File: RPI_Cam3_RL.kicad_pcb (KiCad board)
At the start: 2 copper layers, 106 x 106 mm, 42 parts, among them J1 in, Q1 2N7002, U1 RPI_CAM_3

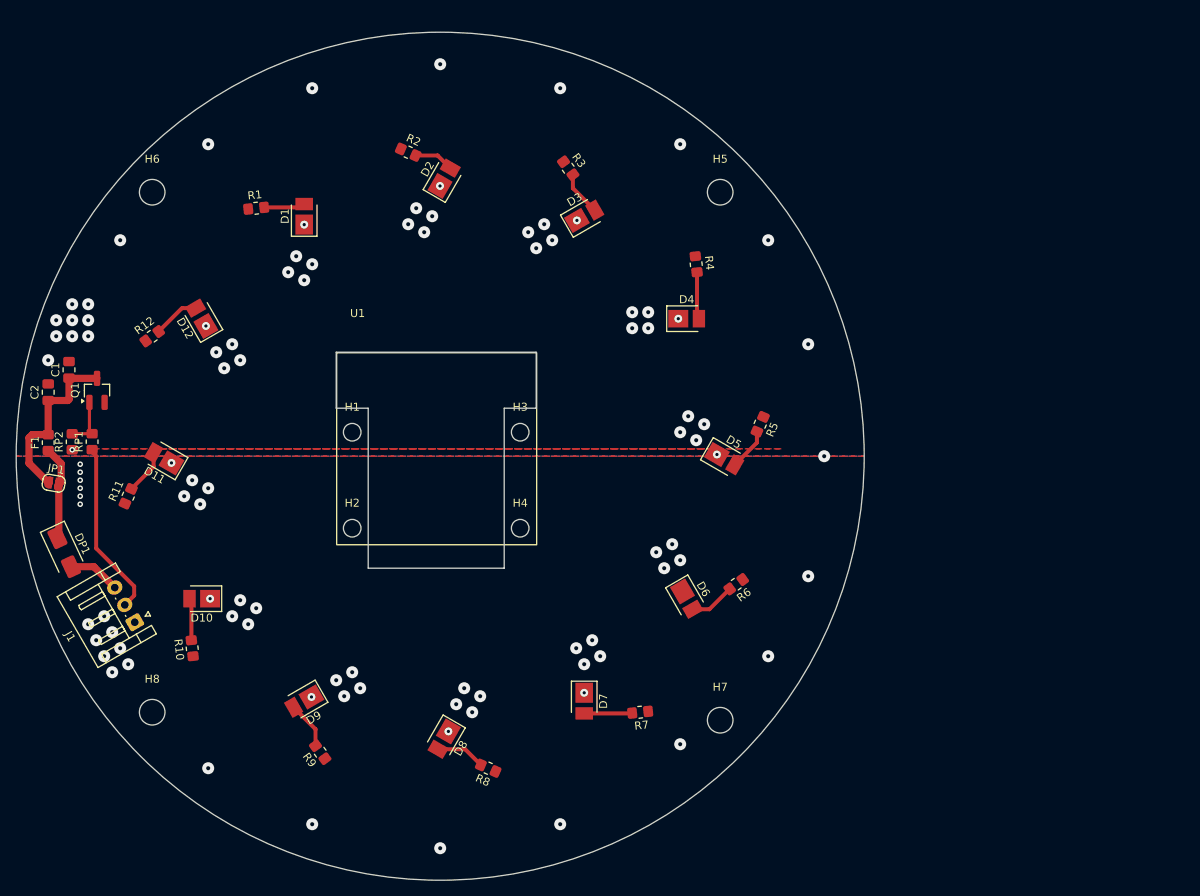
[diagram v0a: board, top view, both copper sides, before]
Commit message: Updated Pcb Design -Small Radius
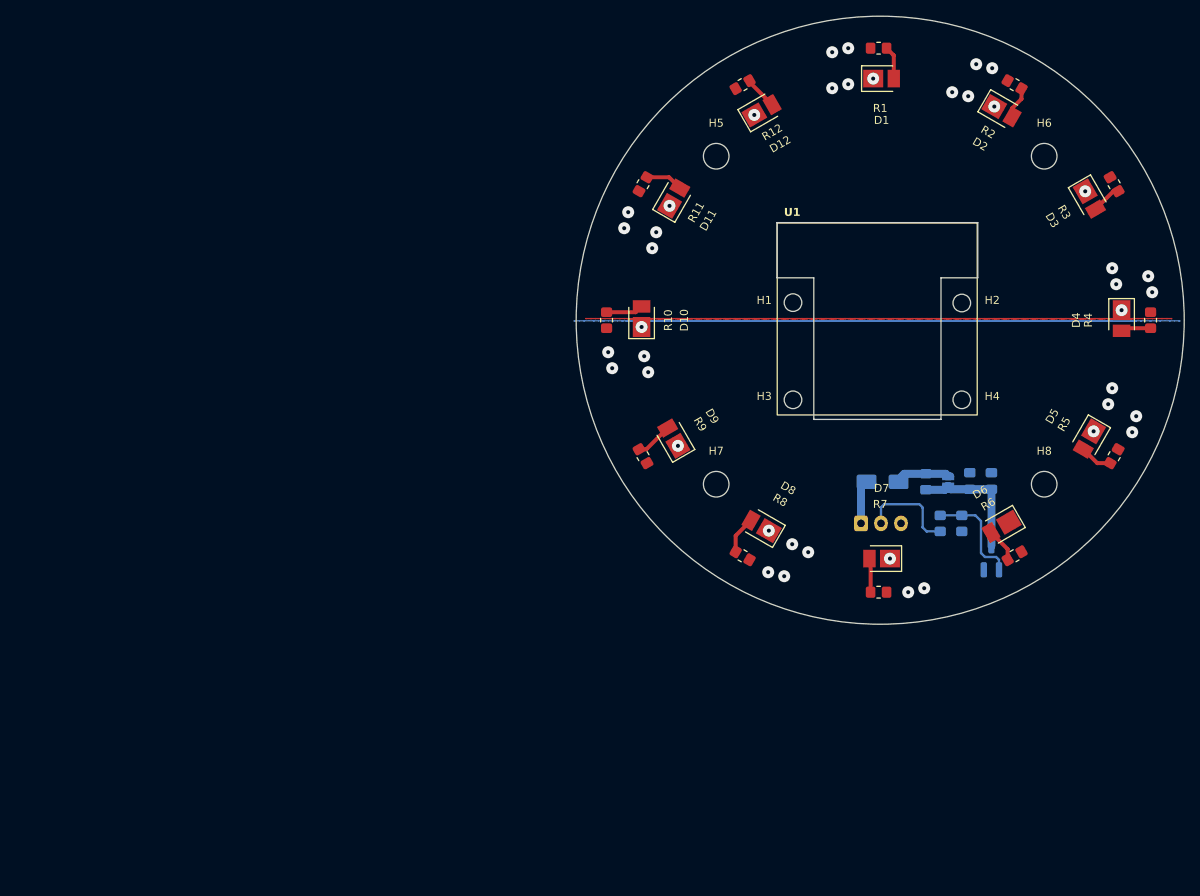
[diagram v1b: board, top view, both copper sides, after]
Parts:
- C1, C2, DP1, F1, J1, JP1, Q1, RP1, RP2: moved to B.Cu
- moved C1 116.1 mm to (218.9, 111.1)
- moved C2 115.7 mm to (216.2, 111.1)
- moved H8 115.1 mm to (225.5, 111.5)
- moved Q1 113.7 mm to (218.9, 120.7)
- moved JP1 111.8 mm to (213.5, 111.2), turned to 90 degrees
- moved RP2 111.7 mm to (215.2, 116.4)
- moved H6 111.6 mm to (225.5, 70.5)
- moved F1 109.8 mm to (210.7, 111.2), turned to -90 degrees
- moved RP1 106.5 mm to (212.5, 116.4)
- moved DP1 102.7 mm to (205.3, 111.2), turned to 180 degrees
- moved J1 91.6 mm to (202.6, 116.4), turned to 0 degrees
- moved H2 81.2 mm to (215.2, 88.8)
- moved R1 80.3 mm to (204.8, 57.0), turned to 0 degrees
- moved R12 80.2 mm to (187.8, 61.6), turned to 30 degrees
- moved R2 76.3 mm to (221.8, 61.6), turned to -30 degrees
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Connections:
- J1 pad 1: GND -> +5V
- J1 pad 3: +5V -> GND
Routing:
- net /EN: track 22.1 -> 12.4 mm
- net Net-(Q1-G): track 6.56 -> 13.2 mm
- net Net-(JP1-A): track 22.2 -> 15.6 mm
- net Net-(DP1-K): track 11.7 -> 6.91 mm
- net Net-(D4-A): track 5.91 -> 3.76 mm
- net Net-(D3-A): track 5.56 -> 3.76 mm
- net Net-(D7-A): track 6.02 -> 4.27 mm
- net Net-(D12-A): track 5.83 -> 4.17 mm
- net Net-(D8-A): track 6.16 -> 4.73 mm
- net Net-(D6-A): track 5.67 -> 4.27 mm
- net Net-(D9-A): track 5.94 -> 4.68 mm
- net Net-(D5-A): track 5.31 -> 4.08 mm
- net +5V: track 6.55 -> 5.49 mm
- net Net-(D11-A): track 5.69 -> 4.66 mm
- net Net-(D1-A): track 5.18 -> 4.17 mm
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- added copper zone on B.Cu, net Net-(Q1-S)
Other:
- board size 106 x 106 mm -> 76 x 76 mm
